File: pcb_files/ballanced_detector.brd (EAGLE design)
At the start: 30.5 x 54.3 mm, 70 parts, among them T1 TCM2-33X+, U1 HMC539ALP3EHCP_16_1_ADI-M, U2 ADA4961ACPZN-R7CP_24_7_ADI-M, U3 HMC539ALP3EHCP_16_1_ADI-M, U4 STM32L051K8T6LQFP32_7X7X1P4-M, U5 AS179-92LFSC70-6_SKY-M, U6 Value, U7 ADL8111ACCZNIC28_ADL8111ACCZN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, U8 TL7660CDGKTDGK8-M

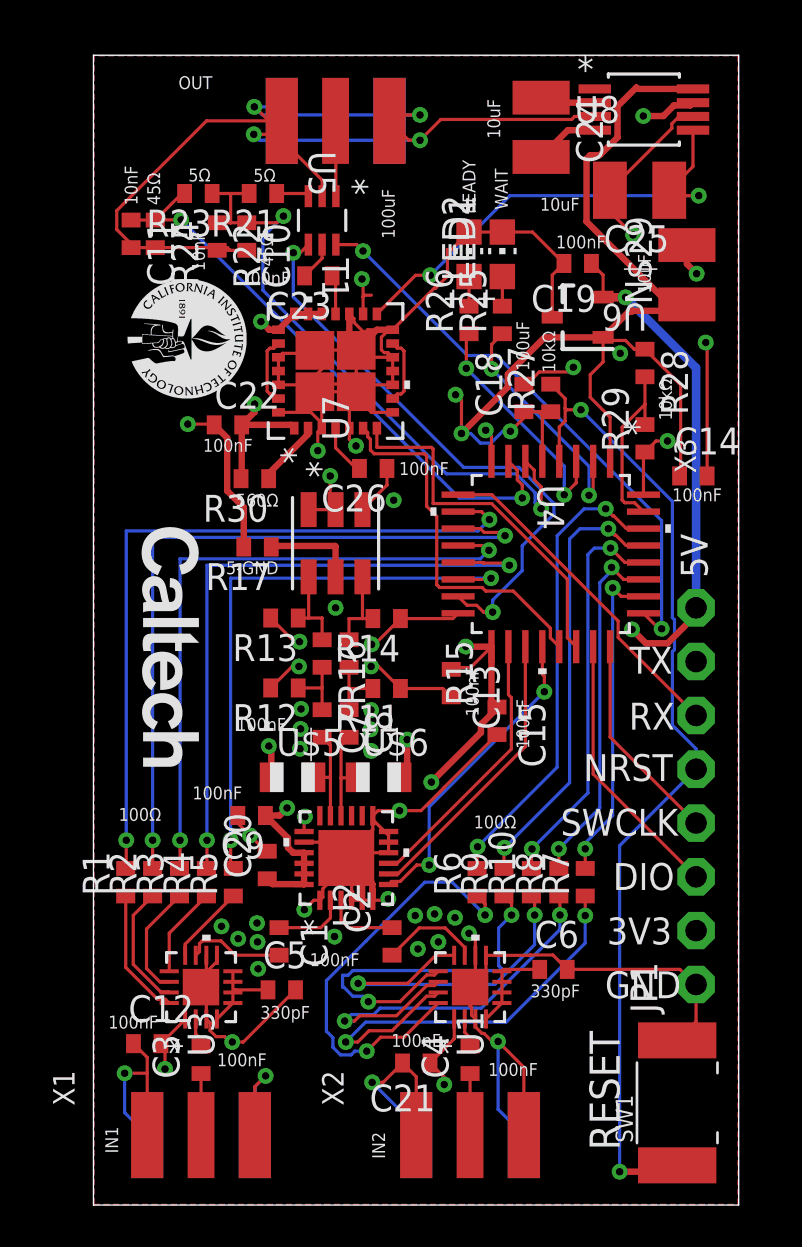
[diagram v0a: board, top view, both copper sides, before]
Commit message: push before reboot
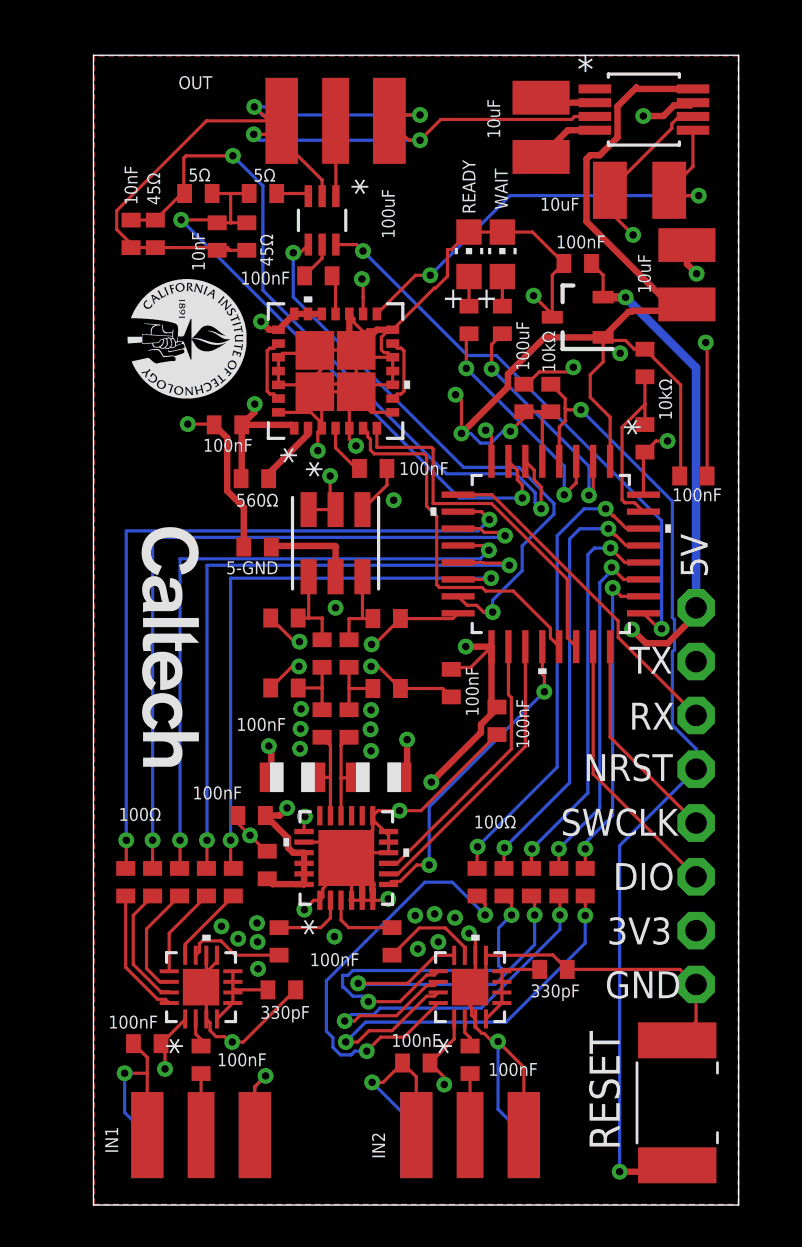
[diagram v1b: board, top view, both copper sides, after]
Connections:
- net ADC1: now also C11.1, R23.2, R24.1; no longer C10.1, R21.2, R22.1, R23.1
- net ADC2: now also C10.1, R21.2, R22.1, R23.1; no longer C11.1, R23.2, R24.1
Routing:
- net ADC1: track 30.5 -> 34.2 mm
- net ADC2: track 27.8 -> 29.8 mm
- net GND: track 381.8 -> 383.1 mm, vias 46 -> 47
- net 3V3: track 109.2 -> 108.6 mm
